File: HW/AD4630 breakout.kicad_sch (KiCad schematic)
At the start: 5 parts, among them U1 AD4630-24BBCZ, U2 AMS1117-1.8, U3 TXS0108EPW, U4 TXS0108EPW, U5 Pico

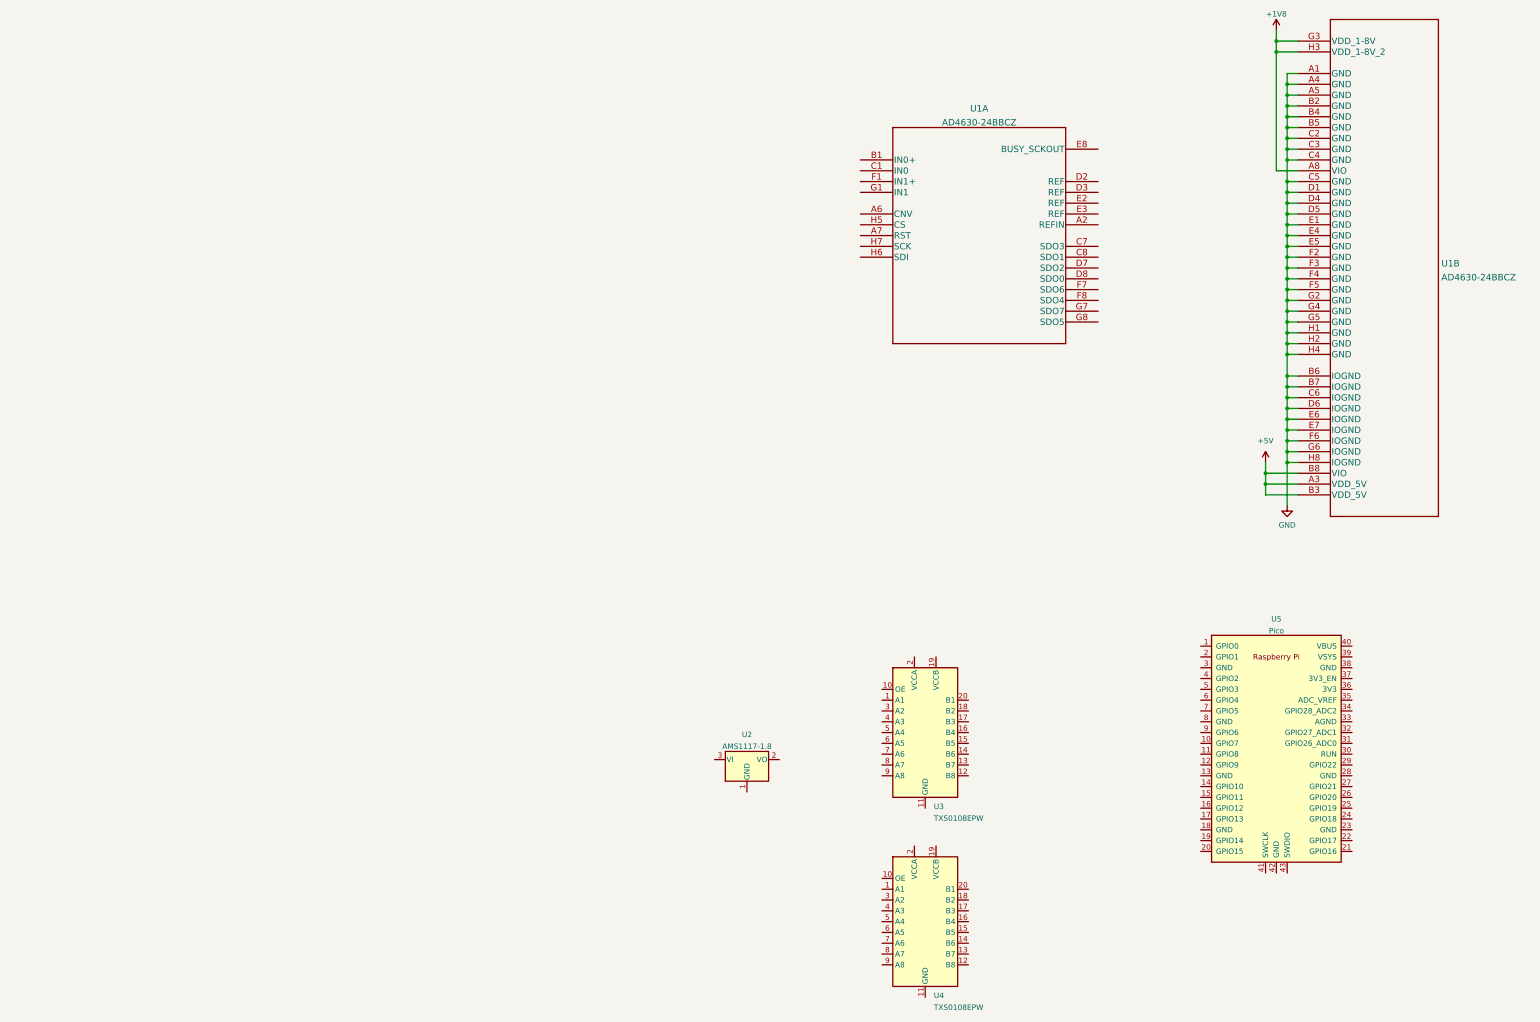
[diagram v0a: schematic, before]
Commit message: PCB updated
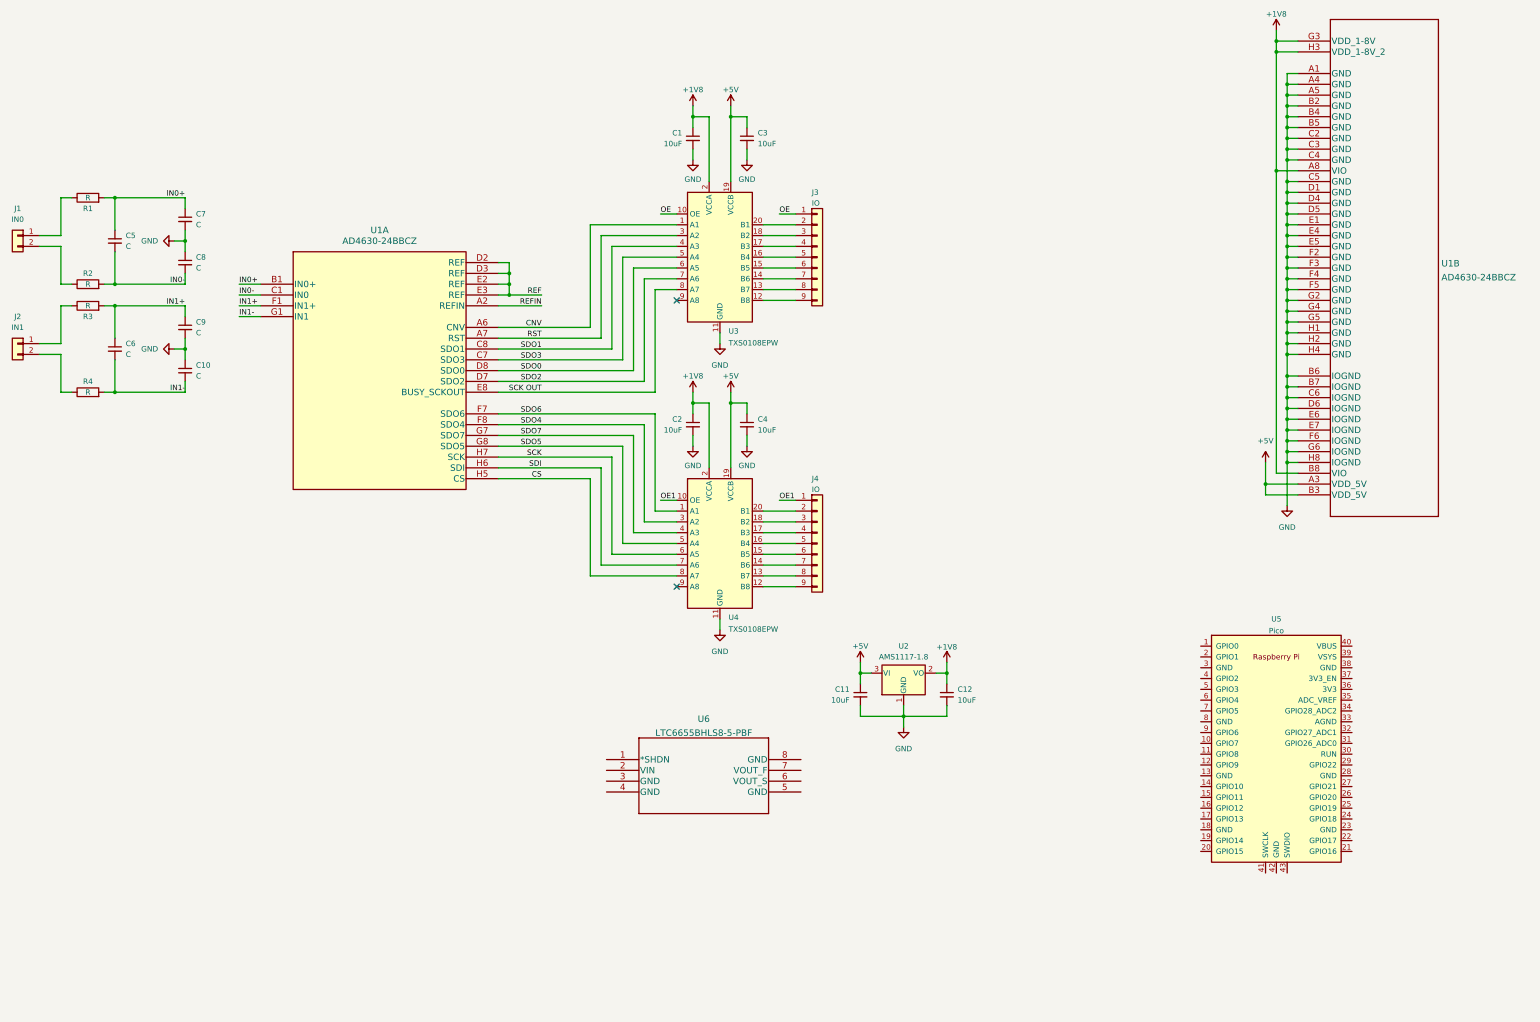
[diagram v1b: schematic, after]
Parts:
- added C1, C11, C12, C2, C3, C4: 10uF, Capacitor_SMD:C_0603_1608Metric, symbol Device:C_Small
- added C10, C5, C6, C7, C8, C9: C, Capacitor_SMD:C_0603_1608Metric, symbol Device:C_Small
- added J1: IN0, Connector_PinHeader_2.54mm:PinHeader_1x02_P2.54mm_Vertical, symbol Connector_Generic:Conn_01x02
- added J2: IN1, Connector_PinHeader_2.54mm:PinHeader_1x02_P2.54mm_Vertical, symbol Connector_Generic:Conn_01x02
- added J3, J4: IO, Connector_PinHeader_2.54mm:PinHeader_1x09_P2.54mm_Vertical, symbol Connector_Generic:Conn_01x09
- added R1, R2, R3, R4: R, Resistor_SMD:R_0603_1608Metric, symbol Device:R
- added U6: LTC6655BHLS8-5-PBF, LTC6655:LTC6655BHLS8-5-PBF, symbol LTC6655:LTC6655BHLS8-5-PBF
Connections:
- net +1V8: now also U1.B8 (VIO), U2.2 (VO), U3.2 (VCCA), U4.2 (VCCA), C1.1, C12.1, C2.1
- net +5V: now also U2.3 (VI), U3.19 (VCCB), U4.19 (VCCB), C11.1, C3.1, C4.1; no longer U1.B8 (VIO)
- net GND: now also U2.1 (GND), U3.11 (GND), U4.11 (GND), C1.2, C10.1, C11.2, C12.2, C2.2, C3.2, C4.2, C7.2, C8.1, C9.2
- net SDO6: now reaches U4.1 (A1)
- net SDO6: now also U1.F7 (SDO6)
- net OE1: now reaches U4.10 (OE)
- net OE1: now also J4.1 (Pin_1)
- net at U4.12 (B8): now also J4.9 (Pin_9)
- net at U4.13 (B7): now also J4.8 (Pin_8)
- net at U4.14 (B6): now also J4.7 (Pin_7)
- net at U4.15 (B5): now also J4.6 (Pin_6)
- net at U4.16 (B4): now also J4.5 (Pin_5)
- net at U4.17 (B3): now also J4.4 (Pin_4)
- net at U4.18 (B2): now also J4.3 (Pin_3)
- net at U4.20 (B1): now also J4.2 (Pin_2)
- net SDO4: now reaches U4.3 (A2)
- net SDO4: now also U1.F8 (SDO4)
- net SDO7: now reaches U4.4 (A3)
- net SDO7: now also U1.G7 (SDO7)
- net SDO5: now reaches U4.5 (A4)
- net SDO5: now also U1.G8 (SDO5)
- net SCK: now reaches U4.6 (A5)
- net SCK: now also U1.H7 (SCK)
- net SDI: now reaches U4.7 (A6)
- net SDI: now also U1.H6 (SDI)
- net CS: now reaches U4.8 (A7)
- net CS: now also U1.H5 (CS)
- net REFIN: now reaches U1.A2 (REFIN)
- net CNV: now reaches U1.A6 (CNV)
- net CNV: now also U3.1 (A1)
- net RST: now reaches U1.A7 (RST)
- net RST: now also U3.3 (A2)
- net IN0+: now reaches U1.B1 (IN0+)
- net IN0+: now also C5.1, C7.1, R1.2
- net IN0-: now reaches U1.C1 (IN0)
- net IN0-: now also C5.2, C8.2, R2.2
- net SDO3: now reaches U1.C7 (SDO3)
- net SDO3: now also U3.5 (A4)
- net SDO1: now reaches U1.C8 (SDO1)
- net SDO1: now also U3.4 (A3)
- net REF: now reaches U1.D2 (REF)
- net REF: now also U1.D3 (REF), U1.E2 (REF), U1.E3 (REF)
- net SDO2: now reaches U1.D7 (SDO2)
- net SDO2: now also U3.7 (A6)
- net SDO0: now reaches U1.D8 (SDO0)
- net SDO0: now also U3.6 (A5)
- net SCK OUT: now reaches U1.E8 (BUSY_SCKOUT)
- net SCK OUT: now also U3.8 (A7)
- net IN1+: now reaches U1.F1 (IN1+)
- net IN1+: now also C6.1, C9.1, R3.2
- net IN1-: now reaches U1.G1 (IN1)
- net IN1-: now also C10.2, C6.2, R4.2
- net OE: now reaches U3.10 (OE)
- net OE: now also J3.1 (Pin_1)
- net at U3.12 (B8): now also J3.9 (Pin_9)
- net at U3.13 (B7): now also J3.8 (Pin_8)
- net at U3.14 (B6): now also J3.7 (Pin_7)
- net at U3.15 (B5): now also J3.6 (Pin_6)
- net at U3.16 (B4): now also J3.5 (Pin_5)
- net at U3.17 (B3): now also J3.4 (Pin_4)
- net at U3.18 (B2): now also J3.3 (Pin_3)
- net at U3.20 (B1): now also J3.2 (Pin_2)
- new net: J2.2 (Pin_2), R4.1
- new net: J1.1 (Pin_1), R1.1
- new net: J1.2 (Pin_2), R2.1
- new net: J2.1 (Pin_1), R3.1
- no-connect marks 0 -> 2
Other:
- moved on the sheet: U2, U3, U4
